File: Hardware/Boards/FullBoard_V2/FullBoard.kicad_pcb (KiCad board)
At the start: 2 copper layers, 153.9 x 70.1 mm, 18 parts, among them J1 Conn_01x03_Pin, J2 Conn_01x03_Pin, J3 Conn_01x03_Pin, J4 Conn_01x03_Pin, K1 Relay_SPDT, U1 GY-8511 UV sensor, U2 TEMT6000, U4 DS18B20-air, U5 DS18B20-water, U6 Turbidity sensor, U7 Water Level

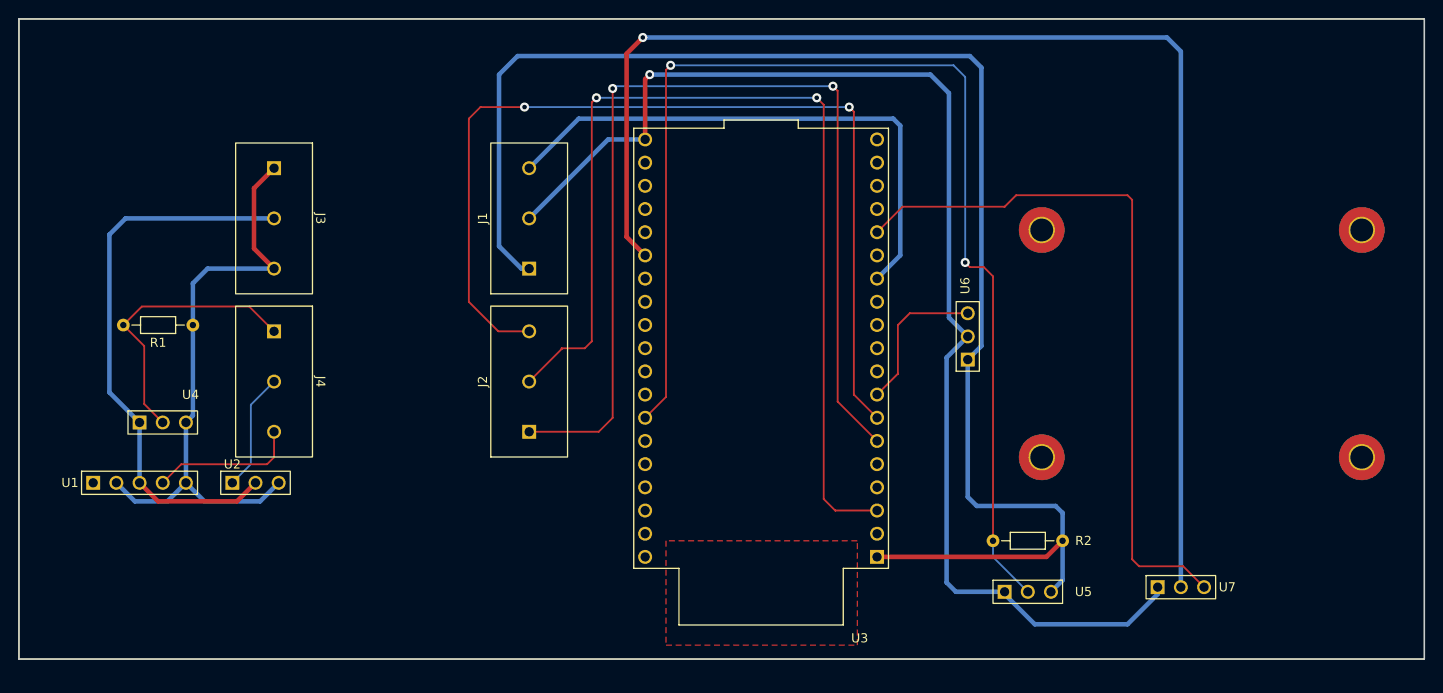
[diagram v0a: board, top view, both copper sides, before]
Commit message: Second version of the full board
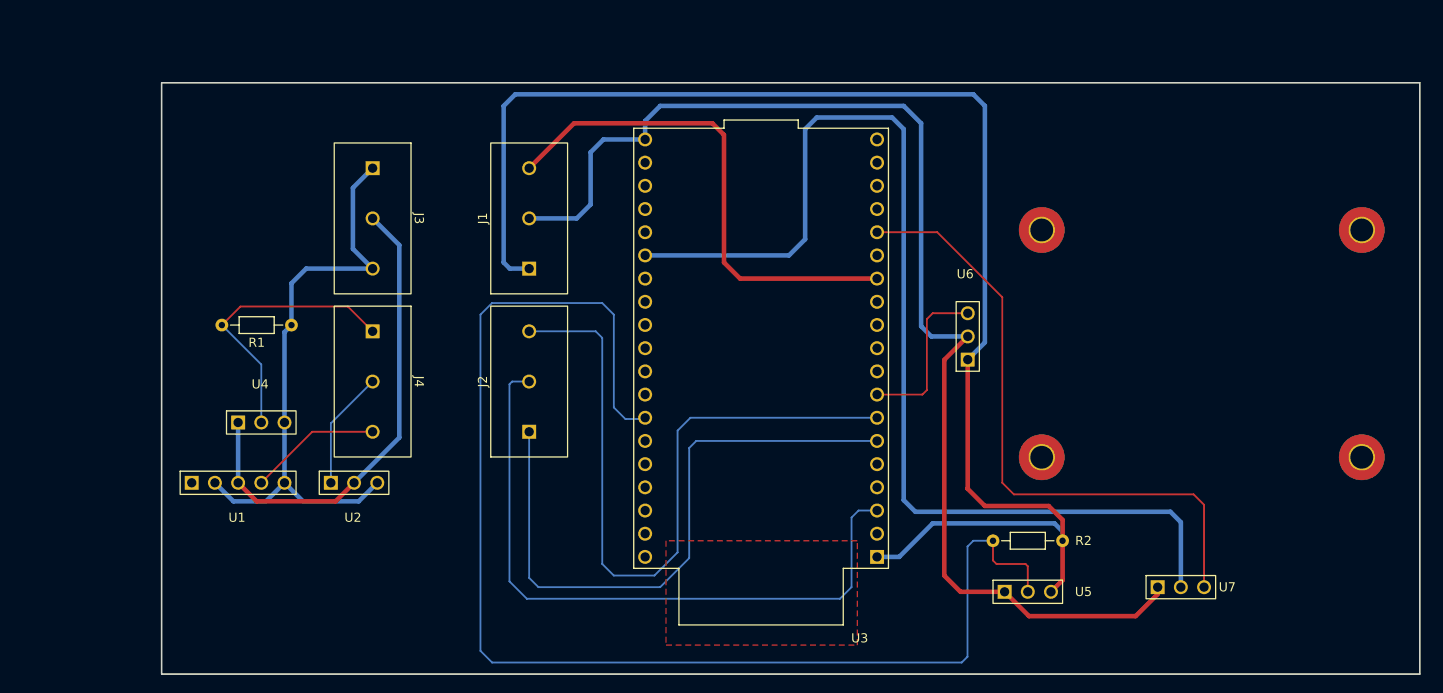
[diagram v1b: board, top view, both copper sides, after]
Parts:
- moved R1 10.8 mm to (74.5, 74.2)
- moved U1 10.8 mm to (78.9, 97.2)
- moved U2 10.8 mm to (86.5, 94.0)
- moved U4 10.8 mm to (76.3, 87.4)
- moved J3 10.8 mm to (83.4, 62.5)
- moved J4 10.8 mm to (83.4, 80.4)
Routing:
- net /Temp_Air: track 110.9 -> 68.2 mm, vias 2 -> 0
- net /Brightness: track 110.4 -> 73.4 mm, vias 2 -> 0
- net /UV: track 105.5 -> 78.7 mm, vias 2 -> 0
- net /Water level Power: track 143.7 -> 121.3 mm, vias 1 -> 0
- net /WaterTemp: track 132.7 -> 144.9 mm, vias 2 -> 0
- net /Water level: track 78.3 -> 69.1 mm
- net GND1: track 61.7 -> 53.2 mm
- net +3.3V: track 166.3 -> 160.1 mm
- net /UV_ref_main: track 61.0 -> 55.4 mm
- net GND: track 139.9 -> 136.4 mm, vias 1 -> 0
- net /UV_OUT: track 16.1 -> 14.5 mm
- net /Turbidity: track 16.7 -> 18.2 mm
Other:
- board size 153.9 x 70.1 mm -> 137.8 x 64.8 mm
